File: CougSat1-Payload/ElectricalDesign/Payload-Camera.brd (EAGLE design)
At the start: 90.4 x 95.8 mm, 84 parts, among them J2 CougSat Card, U1 AD7291, U10 TXS0102DQM, U11 TXS0102DQM, U12 TXS0102DQM, U13 TXS0102DQM, U14 TXS0102DQM, U15 TXS0102DQM, U2 AD8515, U3 AD8616, U4 AD8515, U5 CD74HC4040M, U6 TPS73250, U7 TPS61220, U8 TCA9535R, U9 TXS0102DQM

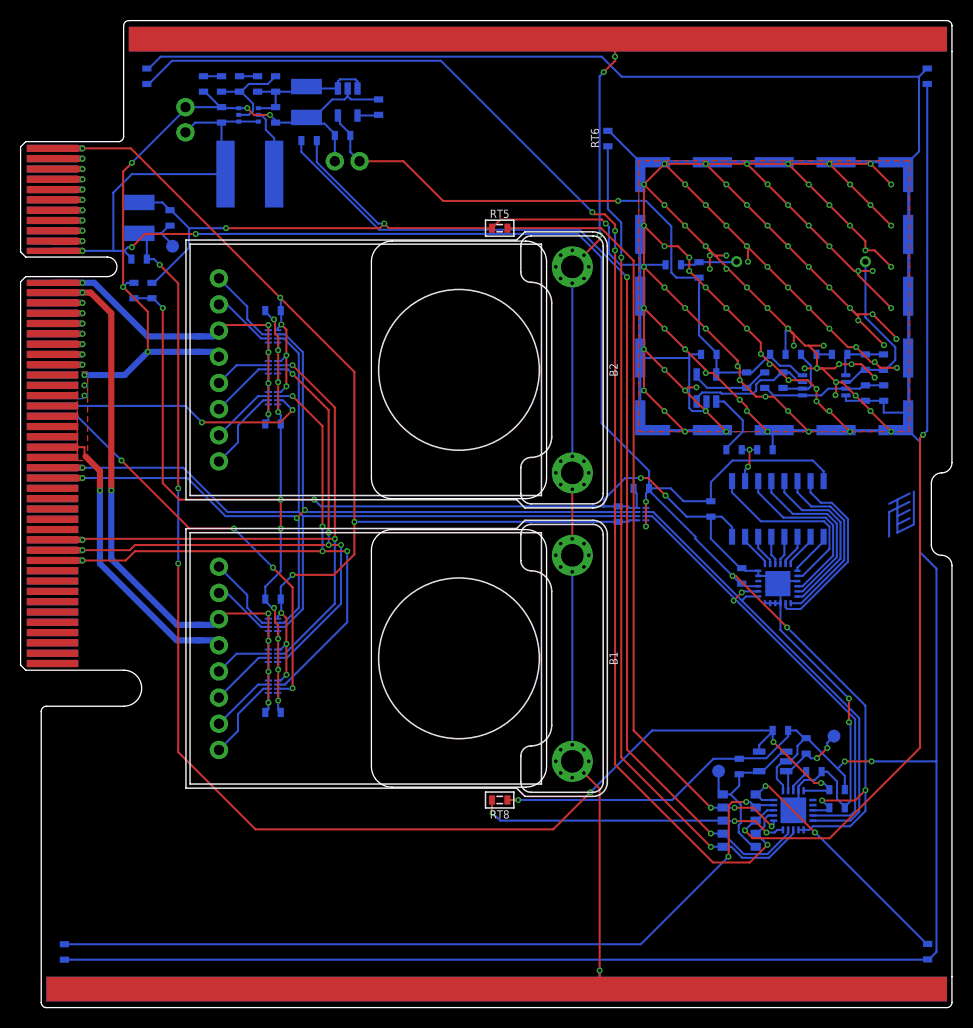
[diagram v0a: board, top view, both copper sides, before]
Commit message: Added balancing
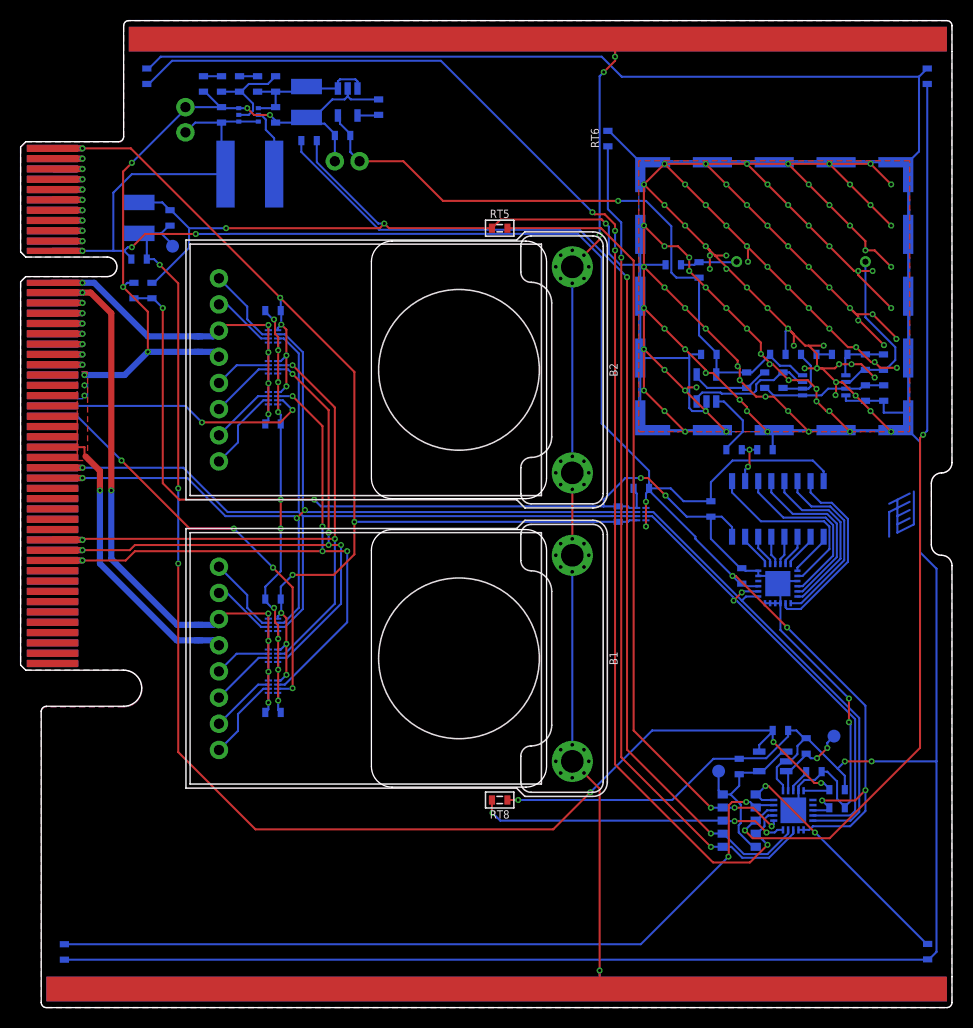
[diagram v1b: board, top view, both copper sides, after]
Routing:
- added copper zone on layer 16, net BALANCING-BOTTOM
- added copper zone on layer 1, net BALANCING-TOP
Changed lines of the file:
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@@
 <drawing>
 <settings>
-<setting alwaysvectorfont="no"/>
+<setting alwaysvectorfont="yes"/>
 <setting verticaltext="up"/>
 </settings>
@@
 </element>
 <element name="J2" library="CougsInSpace-Boards" package="CARD-FULL-OPEN+X" value="CougSat Card" x="7.5" y="50" locked="yes" smashed="yes">
-<attribute name="SKU" value="[Override]" x="7.5" y="50" locked="yes" size="1.778" layer="27" display="off"/>
+<attribute name="SKU" value="68-0007" x="7.5" y="50" locked="yes" size="1.778" layer="27" display="off"/>
 </element>
 </elements>
@@
 <wire x1="87.085" y1="49.23005" x2="85.93505" y2="50.38" width="0.2" layer="16"/>
 </signal>
+<signal name="BALANCING-TOP">
+<polygon width="0.2" layer="1" spacing="0.5" pour="hatch">
+<vertex x="10" y="2.1"/>
+<vertex x="97.4" y="2.1" curve="90"/>
+<vertex x="97.9" y="2.6"/>
+<vertex x="97.9" y="45" curve="90"/>
+<vertex x="96.9" y="46" curve="-90"/>
+<vertex x="95.9" y="47"/>
+<vertex x="95.9" y="53" curve="-90"/>
+<vertex x="96.9" y="54" curve="90"/>
+<vertex x="97.9" y="55"/>
+<vertex x="97.9" y="97.4" curve="90"/>
+<vertex x="97.4" y="97.9"/>
+<vertex x="18" y="97.9" curve="90"/>
+<vertex x="17.5" y="97.4"/>
+<vertex x="17.5" y="86.6" curve="-90"/>
+<vertex x="17" y="86.1"/>
+<vertex x="8" y="86.1"/>
+<vertex x="7.5" y="85.6"/>
+<vertex x="7.5" y="75.45"/>
+<vertex x="8" y="74.95"/>
+<vertex x="15.9" y="74.95" curve="-180"/>
+<vertex x="15.9" y="73.05"/>
+<vertex x="8" y="73.05"/>
+<vertex x="7.5" y="72.55"/>
+<vertex x="7.5" y="35.35"/>
+<vertex x="8" y="34.85"/>
+<vertex x="17.5" y="34.85" curve="-180"/>
+<vertex x="17.5" y="31.3"/>
+<vertex x="10" y="31.3" curve="90"/>
+<vertex x="9.5" y="30.8"/>
+<vertex x="9.5" y="2.6" curve="90"/>
+</polygon>
+</signal>
+<signal name="BALANCING-BOTTOM">
+<polygon width="0.2" layer="16" spacing="0.5" pour="hatch">
+<vertex x="10" y="2.1"/>
+<vertex x="97.4" y="2.1" curve="90"/>
+<vertex x="97.9" y="2.6"/>
+<vertex x="97.9" y="45" curve="90"/>
+<vertex x="96.9" y="46" curve="-90"/>
+<vertex x="95.9" y="47"/>
+<vertex x="95.9" y="53" curve="-90"/>
+<vertex x="96.9" y="54" curve="90"/>
+<vertex x="97.9" y="55"/>
+<vertex x="97.9" y="97.4" curve="90"/>
+<vertex x="97.4" y="97.9"/>
+<vertex x="18" y="97.9" curve="90"/>
+<vertex x="17.5" y="97.4"/>
+<vertex x="17.5" y="86.6" curve="-90"/>
+<vertex x="17" y="86.1"/>
+<vertex x="8" y="86.1"/>
+<vertex x="7.5" y="85.6"/>
+<vertex x="7.5" y="75.45"/>
+<vertex x="8" y="74.95"/>
+<vertex x="15.9" y="74.95" curve="-180"/>
+<vertex x="15.9" y="73.05"/>
+<vertex x="8" y="73.05"/>
+<vertex x="7.5" y="72.55"/>
+<vertex x="7.5" y="35.35"/>
+<vertex x="8" y="34.85"/>
+<vertex x="17.5" y="34.85" curve="-180"/>
+<vertex x="17.5" y="31.3"/>
+<vertex x="10" y="31.3" curve="90"/>
+<vertex x="9.5" y="30.8"/>
+<vertex x="9.5" y="2.6" curve="90"/>
+</polygon>
+</signal>
 </signals>
 <mfgpreviewcolors>
-<mfgpreviewcolor name="soldermaskcolor" color="0xC8008000"/>
-<mfgpreviewcolor name="silkscreencolor" color="0xFFFEFEFE"/>
+<mfgpreviewcolor name="soldermaskcolor" color="0xC8FF0000"/>
+<mfgpreviewcolor name="silkscreencolor" color="0xFFFFFFFF"/>
 <mfgpreviewcolor name="backgroundcolor" color="0xFF282828"/>
 <mfgpreviewcolor name="coppercolor" color="0xFFFFBF00"/>
